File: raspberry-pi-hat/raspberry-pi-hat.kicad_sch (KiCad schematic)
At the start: 7 parts, among them J1 AudioJack3, P1 RaspberryPi-GPIO-header, Q1 PMOS, U1 MCP3204

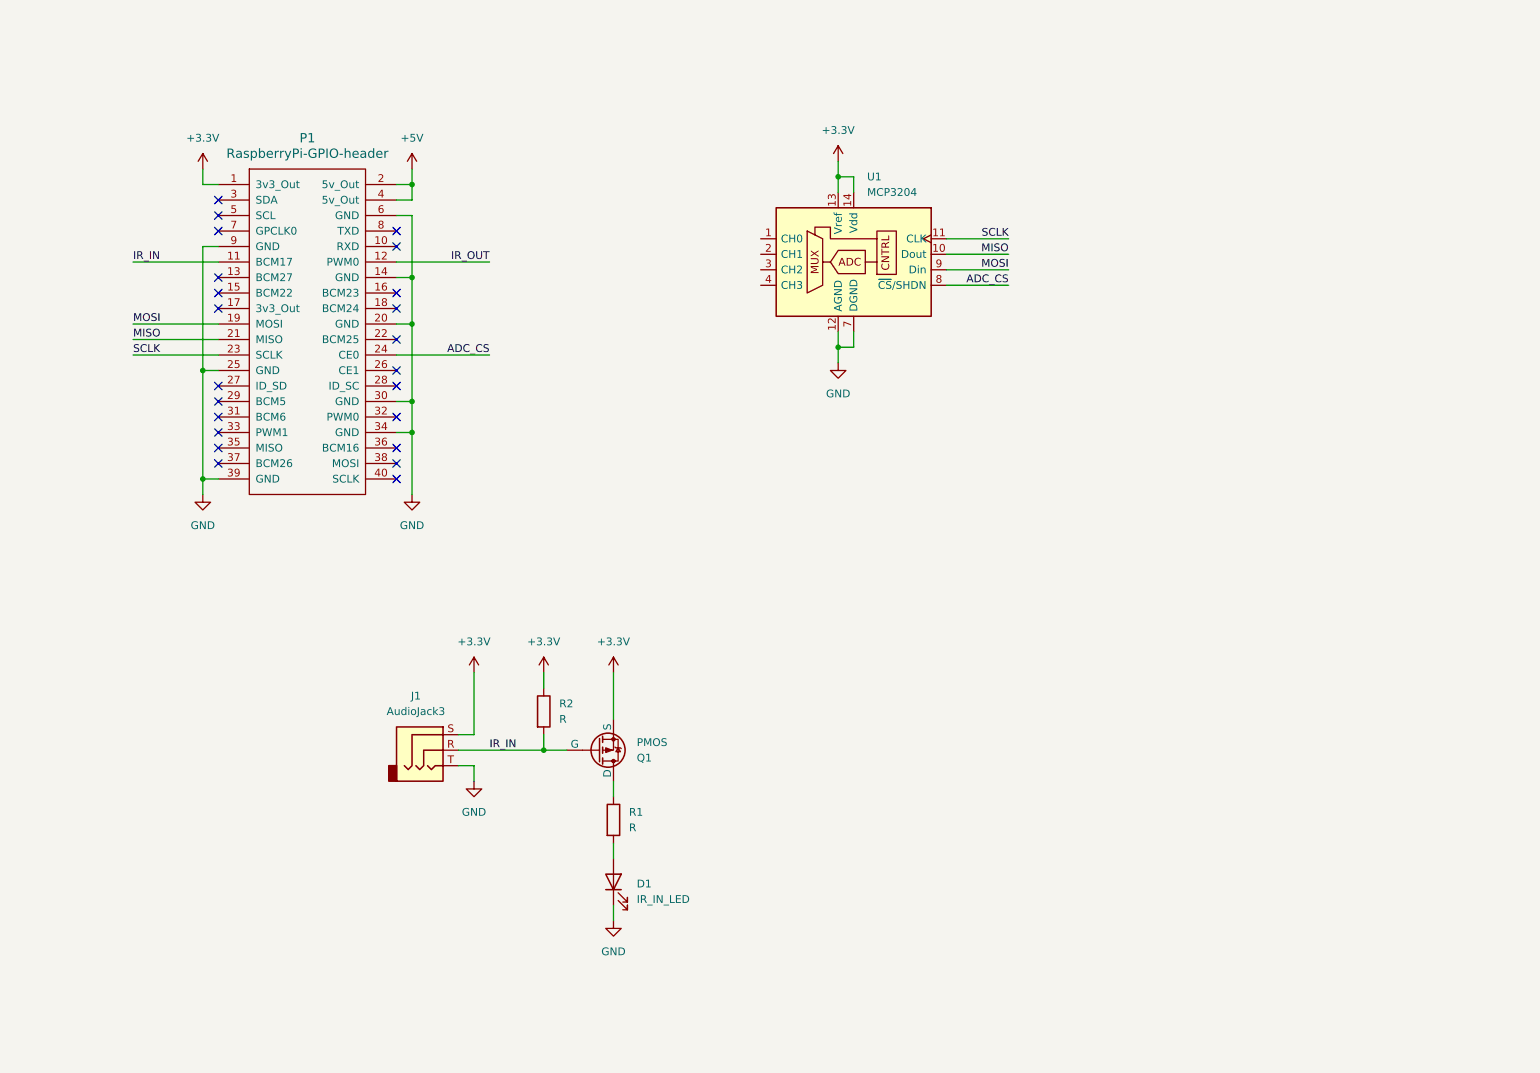
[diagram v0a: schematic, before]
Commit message: initial schematic
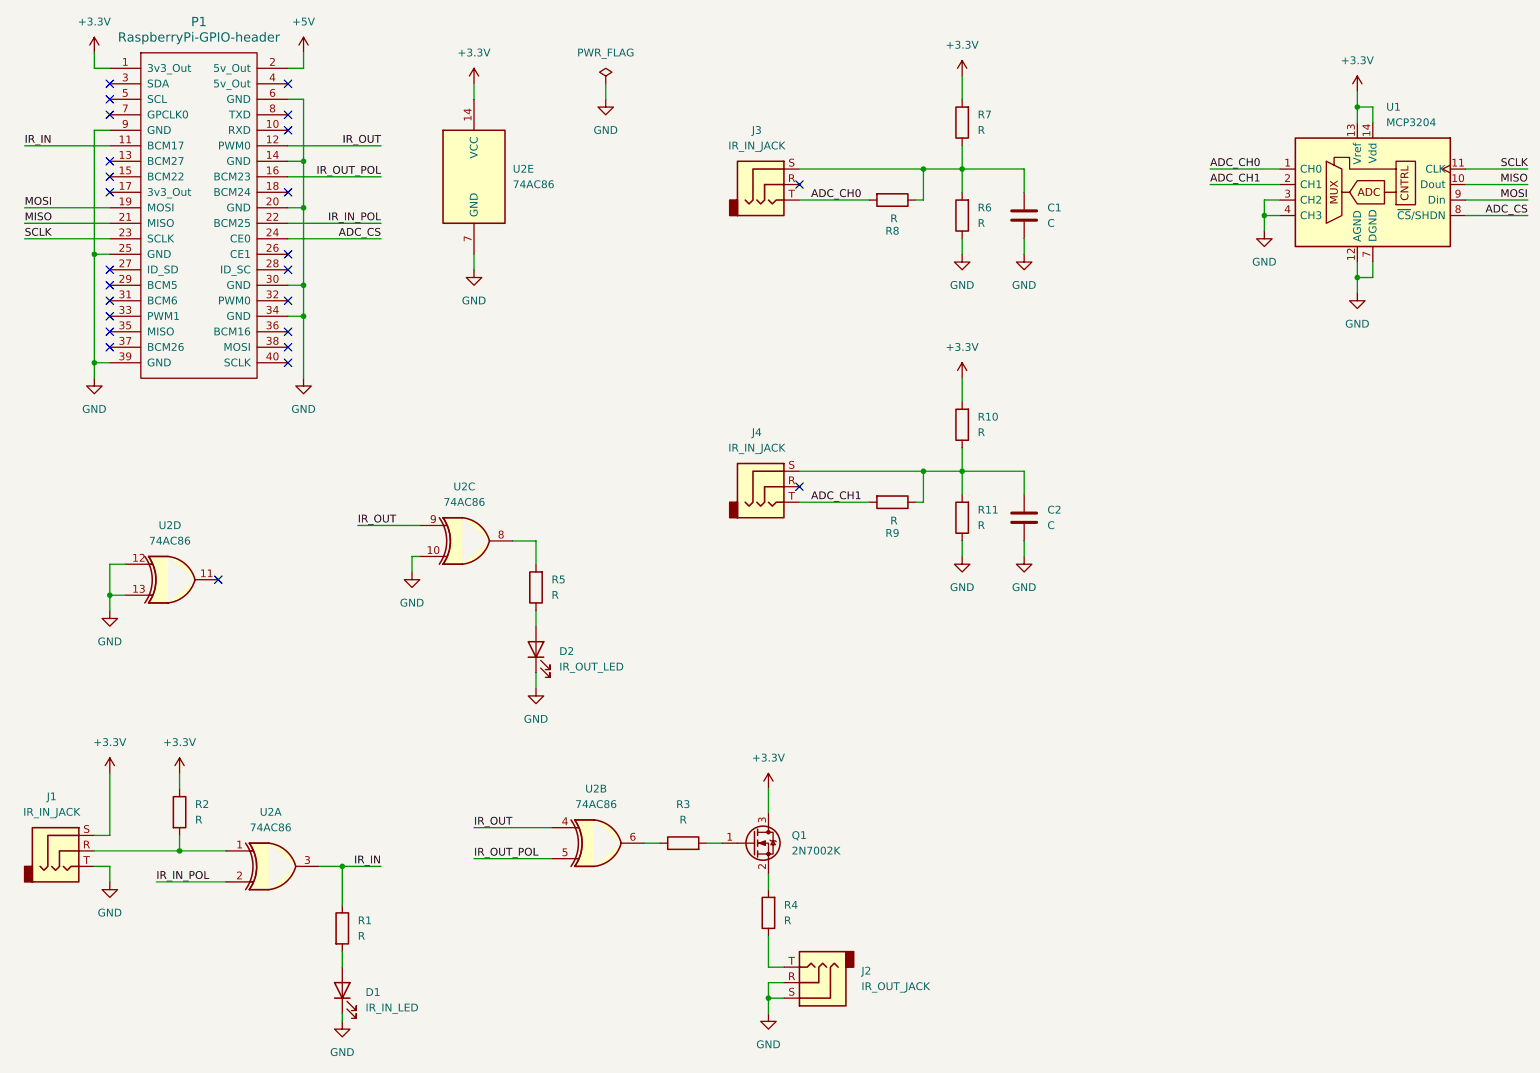
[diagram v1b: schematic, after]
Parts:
- removed Q1: PMOS, symbol Simulation_SPICE:PMOS
- added C1, C2: C, symbol Device:C
- added D2: IR_OUT_LED, symbol Device:LED
- added J2: IR_OUT_JACK, symbol Connector_Audio:AudioJack3
- added J3, J4: IR_IN_JACK, symbol Connector_Audio:AudioJack3
- added Q1: 2N7002K, Package_TO_SOT_SMD:SOT-23, symbol Transistor_FET:2N7002K
- added R10, R11, R3, R4, R5, R6, R7, R8, R9: R, symbol Device:R
- added U2: 74AC86, symbol 74xx:74LS86
- J1: value AudioJack3 -> IR_IN_JACK
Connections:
- net +3.3V: now also Q1.3 (D), R10.2, R7.2, U2.14 (VCC)
- net +5V: no longer P1.4 (5v_Out)
- net GND: now also U1.3 (CH2), U1.4 (CH3), C1.2, C2.2, D2.1 (K), J2.R, J2.S, R11.1, R6.1, U2.10, U2.12, U2.13, U2.7 (GND)
- net IR_IN: now also R1.1, U2.3; no longer J1.R, R2.2
- net IR_OUT: now also U2.4, U2.9
- net IR_OUT_POL: now reaches P1.16 (BCM23)
- net IR_OUT_POL: now also U2.5
- net IR_IN_POL: now reaches P1.22 (BCM25)
- net IR_IN_POL: now also U2.2
- net ADC_CH0: now reaches U1.1 (CH0)
- net ADC_CH0: now also J3.T, R8.2
- net ADC_CH1: now reaches U1.2 (CH1)
- net ADC_CH1: now also J4.T, R9.2
- new net: C1.1, J3.S, R6.2, R7.1, R8.1
- new net: J1.R, R2.2, U2.1
- new net: R3.1, U2.6
- new net: Q1.1 (G), R3.2
- new net: Q1.2 (S), R4.2
- new net: D2.2 (A), R5.1
- new net: R5.2, U2.8
- new net: C2.1, J4.S, R10.1, R11.2, R9.1
- new net: J2.T, R4.1
- no-connect marks 23 -> 25
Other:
- moved on the sheet: D1, J1, P1, R2, U1
